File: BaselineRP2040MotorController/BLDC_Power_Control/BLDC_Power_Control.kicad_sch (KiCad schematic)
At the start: 7 parts, among them J3 Conn_01x03

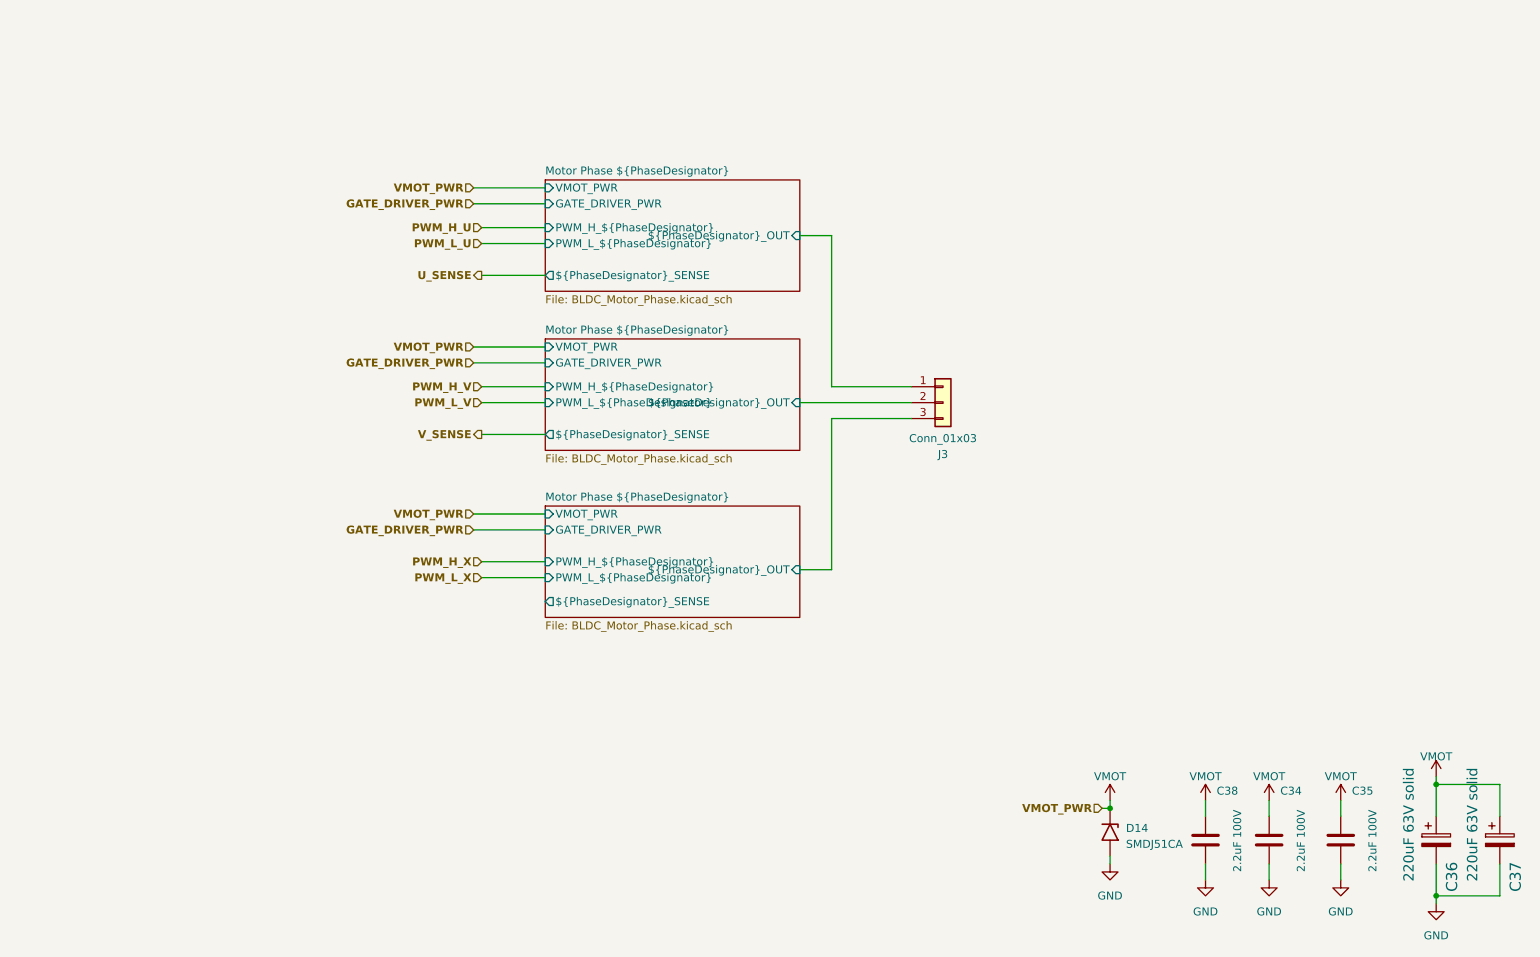
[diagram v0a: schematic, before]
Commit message: Release for Review
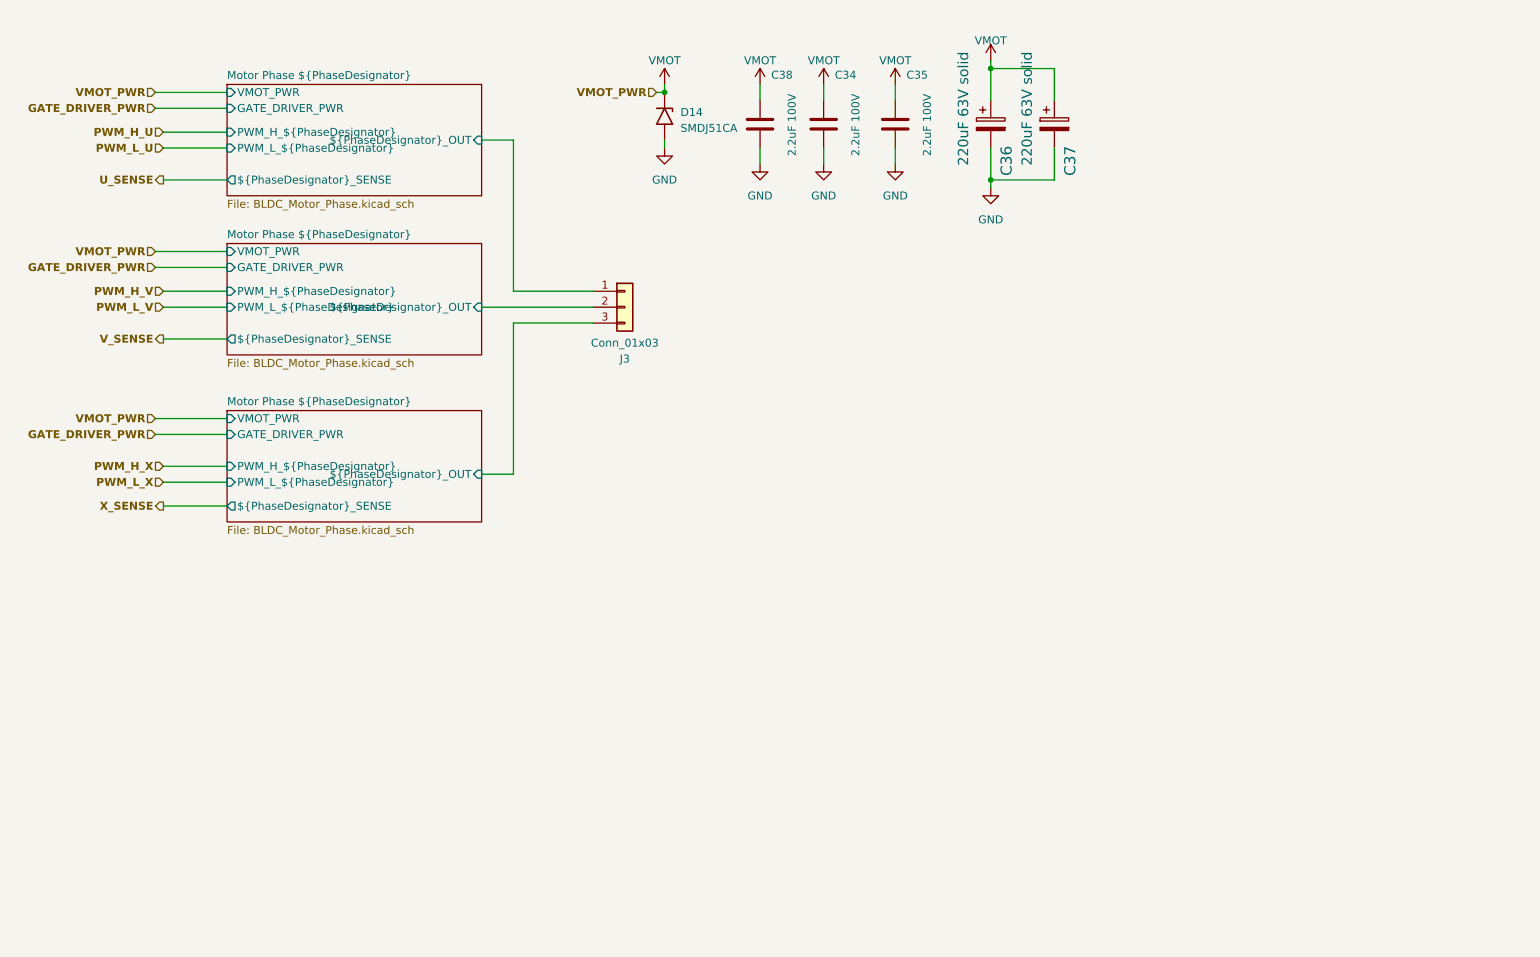
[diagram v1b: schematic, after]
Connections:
- net Motor Phase ${PhaseDesignator}/${PhaseDesignator}_OUT is gone; now on net Motor Phase ${PhaseDesignator}/${PhaseDesignator}_OUT: J3.3 (Pin_3)
- net Motor Phase ${PhaseDesignator}/${PhaseDesignator}_OUT: no longer J3.1 (Pin_1)
- new net Motor Phase ${PhaseDesignator}/${PhaseDesignator}_OUT: J3.1 (Pin_1)
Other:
- moved on the sheet: C34, C35, C36, C37, C38, D14, J3
